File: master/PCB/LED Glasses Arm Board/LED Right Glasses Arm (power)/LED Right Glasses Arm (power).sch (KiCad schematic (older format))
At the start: 27 parts, among them J1 Conn_01x02_Male, J2 Conn_01x01_Male, J3 Conn_01x01_Male, Q1 TP0610T, SW1 SW_SPST, U1 TPS63061DSCT

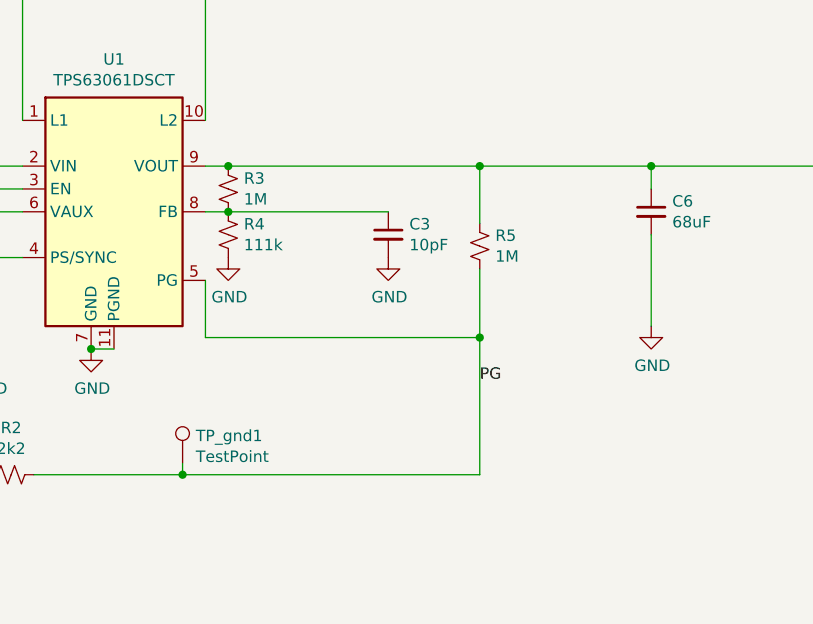
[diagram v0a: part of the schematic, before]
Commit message: updated board
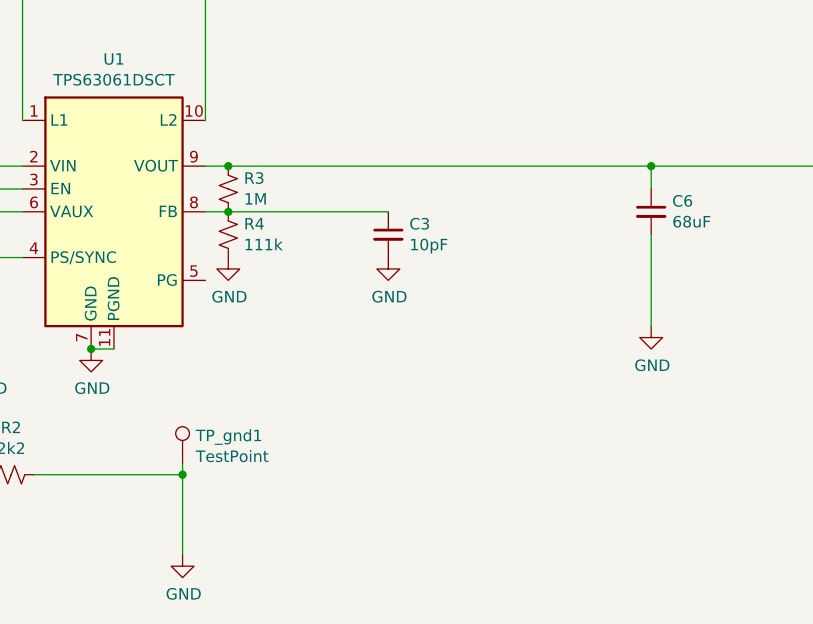
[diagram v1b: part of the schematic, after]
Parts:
- removed R5: 1M, Resistor_SMD:R_0603_1608Metric, symbol Device:R_Small_US
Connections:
- net GND: now also R2.2, TP_gnd1.1
- removed net PG: R2.2, TP_gnd1.1, U1.5 (PG)
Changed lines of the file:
@@
 	5150 3300 5150 3850
-Wire Wire Line
-	5150 4800 6350 4800
 Wire Wire Line
 	5150 4050 5250 4050
@@
 Connection ~ 5250 4050
 Wire Wire Line
-	5250 4050 6350 4050
-Wire Wire Line
 	5150 4250 5250 4250
 $Comp
@@
 	1    0    0    -1
 $EndComp
-Wire Wire Line
-	5150 4550 5150 4800
 $Comp
 L power:GND #PWR0106
@@
 $EndComp
 $Comp
-L Device:R_Small_US R5
-U 1 1 5F4BBDC6
-P 6350 4400
-F 0 "R5" H 6418 4446 50  0000 L CNN
-F 1 "1M" H 6418 4355 50  0000 L CNN
-F 2 "Resistor_SMD:R_0603_1608Metric" H 6350 4400 50  0001 C CNN
-F 3 "https://www.yageo.com/upload/media/product/productsearch/datasheet/rchip/PYu-RT_1-to-0.01_RoHS_L_12.pdf" H 6350 4400 50  0001 C CNN
-F 4 "https://www.digikey.com.au/product-detail/en/yageo/RT0603BRD071ML/YAG4498CT-ND/6616654" H 6350 4400 50  0001 C CNN "Digikey Link"
-	1    6350 4400
-	1    0    0    -1
-$EndComp
-Wire Wire Line
-	6350 4050 6350 4300
-Wire Wire Line
-	6350 4500 6350 4800
-Connection ~ 6350 4050
-$Comp
 L power:GND #PWR0108
 U 1 1 5F4BEA89
@@
 Text Label 8550 4050 0    50   ~ 0
 VOUT_5V
-Connection ~ 6350 4800
-Text Label 6350 5000 0    50   ~ 0
-PG
 Wire Wire Line
 	4350 4150 3700 4150
@@
 Connection ~ 3700 5400
 Wire Wire Line
-	6350 4800 6350 5400
-Wire Wire Line
 	4400 5400 5050 5400
 $Comp
@@
 $EndComp
 Wire Wire Line
-	6350 4050 7100 4050
-Wire Wire Line
 	7100 4050 7100 4150
 Connection ~ 7100 4050
@@
 Wire Wire Line
 	2350 4050 2850 4050
+$Comp
+L power:GND #PWR0112
+U 1 1 6075711B
+P 5050 5750
+F 0 "#PWR0112" H 5050 5500 50  0001 C CNN
+F 1 "GND" H 5055 5577 50  0000 C CNN
+F 2 "" H 5050 5750 50  0001 C CNN
+F 3 "" H 5050 5750 50  0001 C CNN
+	1    5050 5750
+	1    0    0    -1
+$EndComp
 Wire Wire Line
 	5050 5350 5050 5400
 Connection ~ 5050 5400
 Wire Wire Line
-	5050 5400 6350 5400
+	5050 5400 5050 5750
+Wire Wire Line
+	5250 4050 7100 4050
 $EndSCHEMATC
